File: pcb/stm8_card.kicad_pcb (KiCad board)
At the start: 2 copper layers, 101.6 x 50.8 mm, 22 parts, among them J1 DEBUG HEADER, SW1 TL59AF100Q, SW2 TL59AF100Q, SW3 TL59AF100Q, SW4 TL3302AF260QG, U1 ER-OLED0.91-7, U2 STM8S103F3

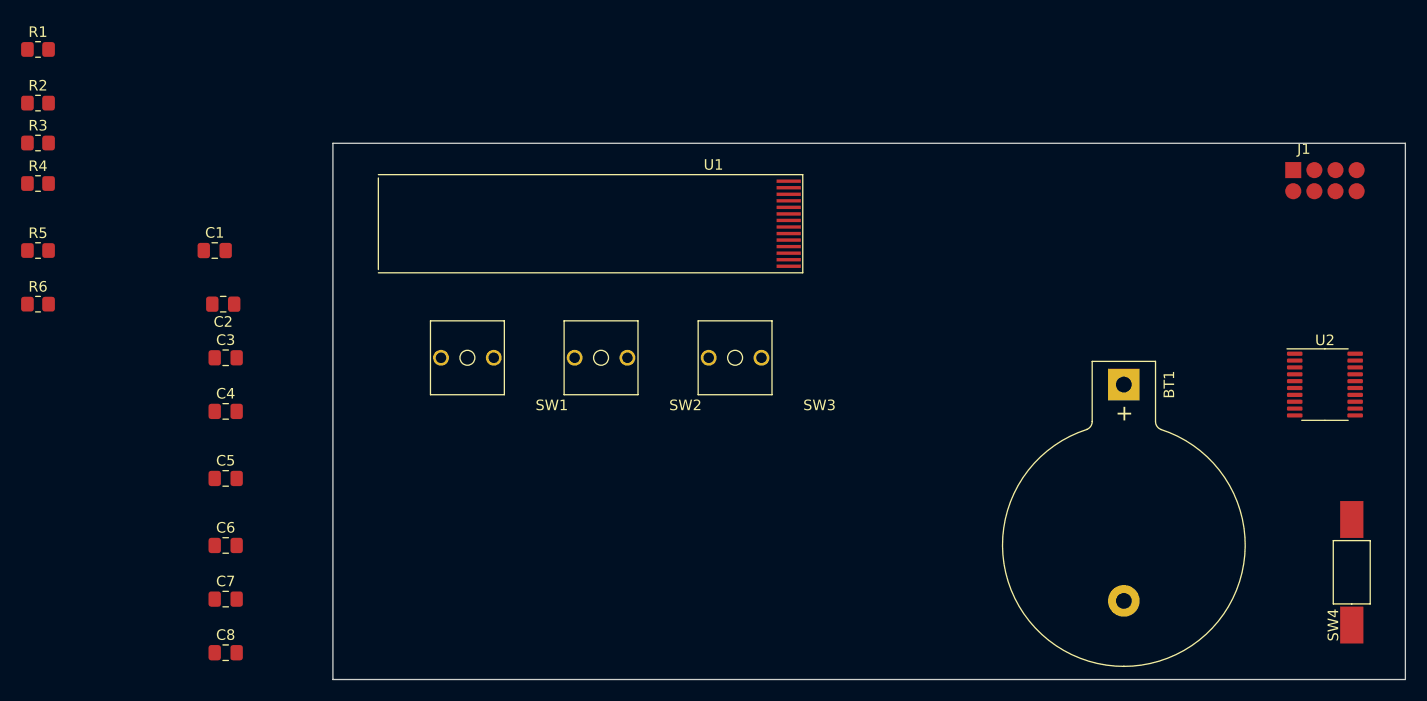
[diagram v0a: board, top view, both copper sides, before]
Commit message: pcbupdates
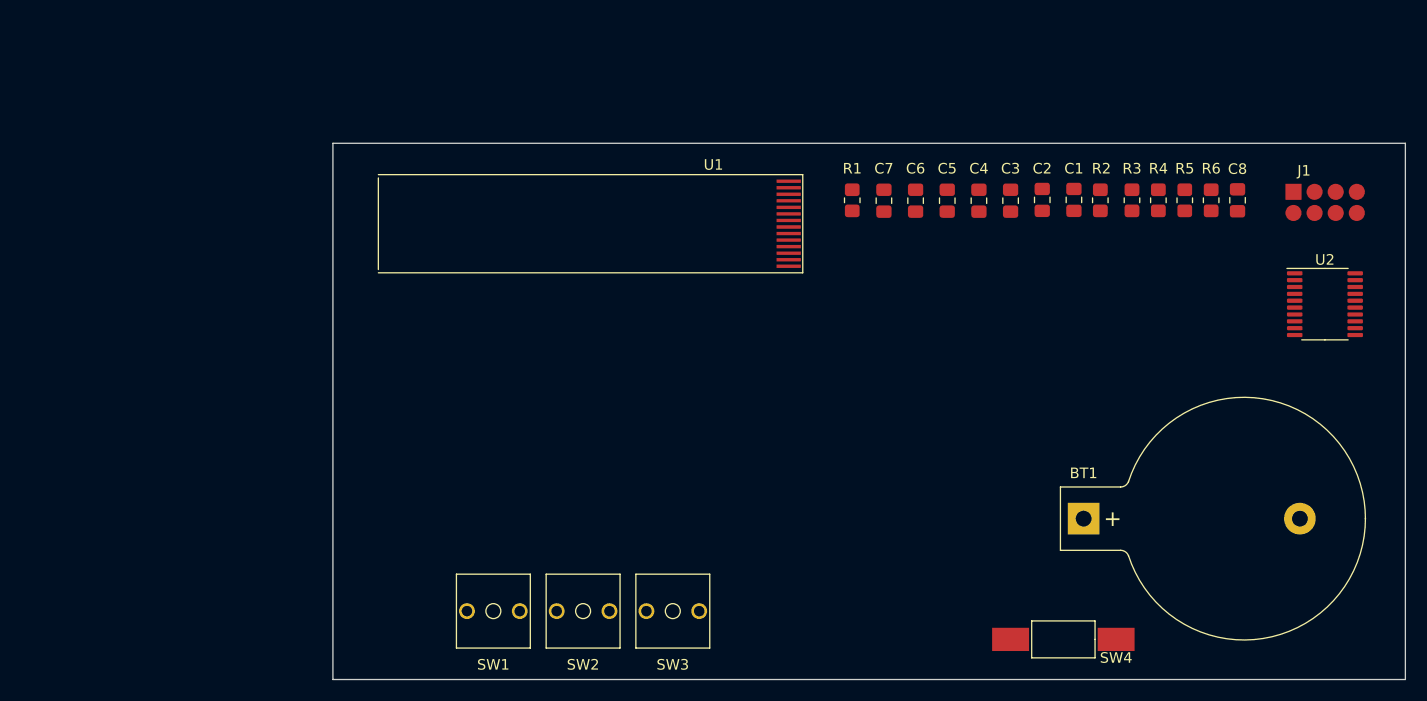
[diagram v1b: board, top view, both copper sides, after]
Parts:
- BT1: footprint Battery:BatteryHolder_Keystone_103_1x20mm -> stm8_card:BatteryHolder_Keystone_103_1x20mm_Corrected
- moved R6 111.6 mm to (261.0, 107.0), turned to 270 degrees
- moved R5 108.7 mm to (258.5, 107.0), turned to 270 degrees
- moved R4 106.2 mm to (256.0, 107.0), turned to 90 degrees
- moved C8 105.0 mm to (263.5, 107.0), turned to 90 degrees
- moved R3 103.8 mm to (253.5, 107.0), turned to 90 degrees
- moved R2 101.1 mm to (250.5, 107.0), turned to 90 degrees
- moved C1 81.5 mm to (248.0, 107.0), turned to 90 degrees
- moved R1 78.5 mm to (227.0, 107.0), turned to 90 degrees
- moved C2 78.2 mm to (245.0, 107.0), turned to 90 degrees
- moved C3 75.8 mm to (242.0, 107.0), turned to 90 degrees
- moved C4 74.1 mm to (239.0, 107.0), turned to 90 degrees
- moved C5 73.2 mm to (236.0, 107.0), turned to 270 degrees
- moved C6 73.1 mm to (233.0, 107.0), turned to 270 degrees
- moved C7 72.9 mm to (230.0, 107.0), turned to 270 degrees
- moved SW4 28.1 mm to (247.0, 148.6), turned to 180 degrees
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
